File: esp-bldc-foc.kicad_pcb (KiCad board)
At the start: 4 copper layers, 66 x 66 mm, 94 parts, among them IC1 ESP32-S3FN8, IC2 LY68L6400SLIT, IC3 AS5600-ASOM, J1 USB_C_Receptacle_USB2.0, J10 UART, J3 I2C ENCODER, J6 Conn_01x02_Female, J7 A, J8 B, J9 C, Q1 BUK7M9R9-60EX, Q10 BUK7M9R9-60EX, Q11 BUK7M9R9-60EX, Q12 BUK7M9R9-60EX, Q2 BUK7M9R9-60EX, Q3 BUK7M9R9-60EX, Q4 BUK7M9R9-60EX, Q5 BUK7M9R9-60EX, Q6 BUK7M9R9-60EX, Q7 BUK7M9R9-60EX, Q8 BUK7M9R9-60EX, Q9 BUK7M9R9-60EX, SW1 SW_SPST, SW2 SW_SPST, U1 NCP163ASN330T1G, U2 DRV8353SMRTAT, U5 LMR36510ADDA, Y1 40MHz

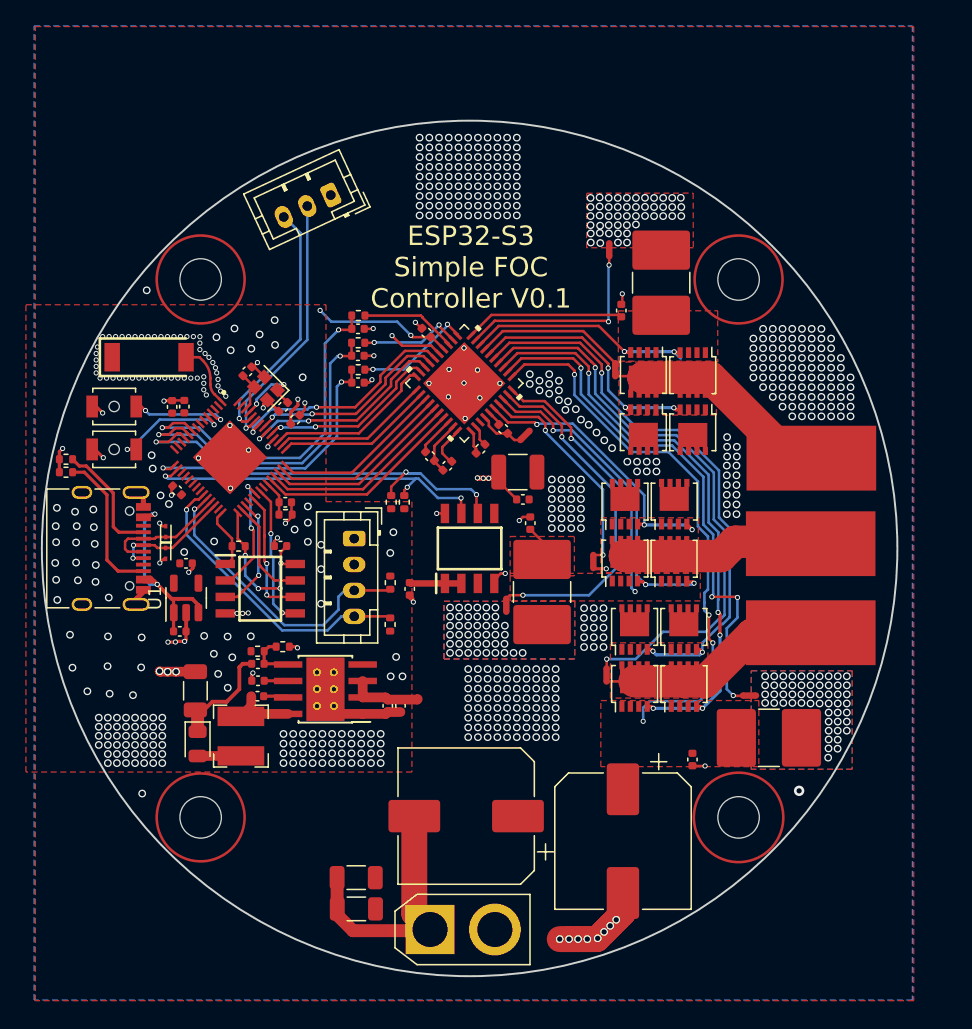
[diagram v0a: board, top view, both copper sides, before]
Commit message: init routing done
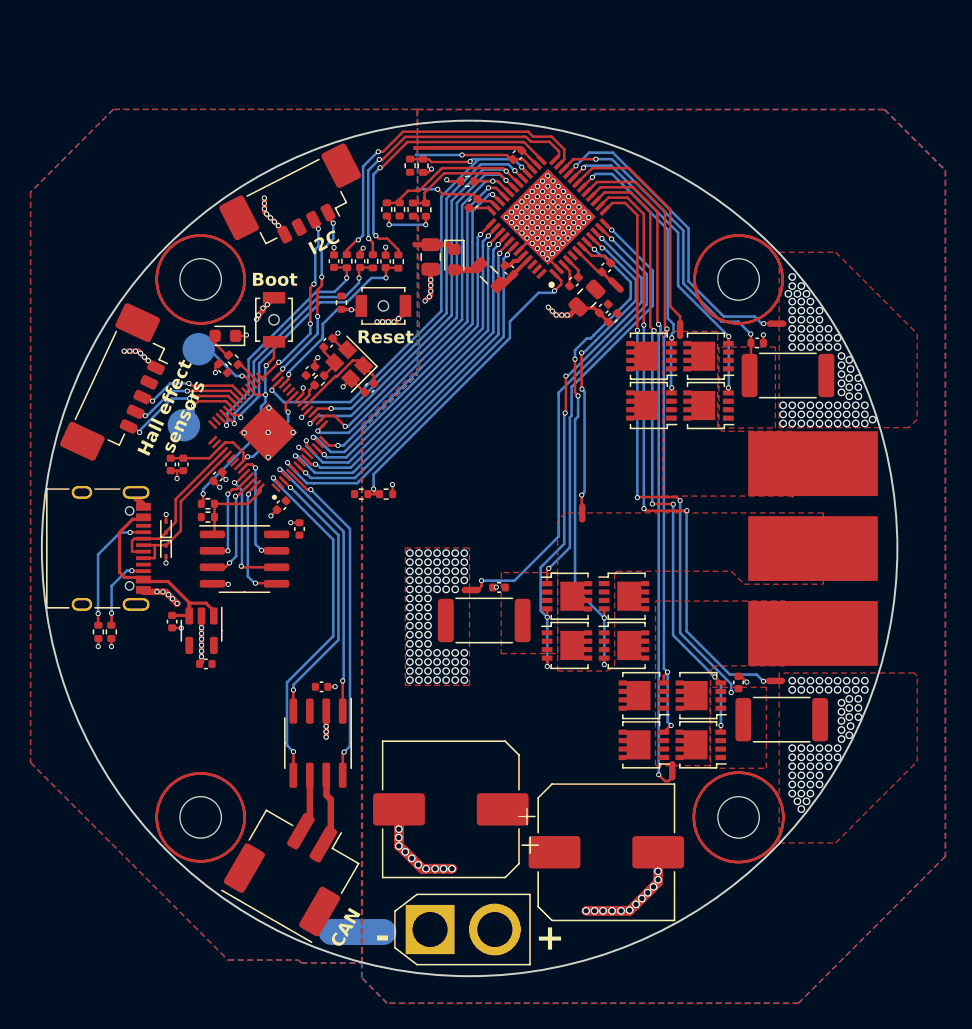
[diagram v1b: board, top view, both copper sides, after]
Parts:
- removed AE1: Antenna_Chip, 2450AT43F0100:ANTC6020X130N
- removed C32, C38: 1uF, Capacitor_SMD:C_0402_1005Metric
- removed C34, C36: 220nF, Capacitor_SMD:C_0402_1005Metric
- removed C40: 100nF, Capacitor_SMD:C_0402_1005Metric
- removed C42: 10pF, Capacitor_SMD:C_0402_1005Metric
- removed C44: 47uF, Capacitor_SMD:C_1206_3216Metric
- removed C46: 470uF, Capacitor_SMD:CP_Elec_10x10
- removed C49, C52: 4.7uF, Capacitor_SMD:C_1206_3216Metric
- removed D6: D, Diode_SMD:D_0805_2012Metric
- removed IC3: AS5600-ASOM, AS5600:SOIC127P600X175-8N
- removed J10: UART, Connector_JST:JST_PH_B3B-PH-K_1x03_P2.00mm_Vertical
- removed L4: 22uH, Inductor_SMD:L_Bourns-SRN4018
- removed R10, R11, R12, R9: 10K, Resistor_SMD:R_0402_1005Metric
- removed U5: LMR36510ADDA, Package_SO:Texas_HTSOP-8-1EP_3.9x4.9mm_P1.27mm_EP2.95x4.9mm_Mask2.4x3.1mm_ThermalVias
- added C24: 22uF, Capacitor_SMD:C_0805_2012Metric, F.Cu at (143.6, 78.5)
- added C25: C, Capacitor_SMD:C_0402_1005Metric, F.Cu at (135.2, 111.6)
- added C26: 0.1uF, Capacitor_SMD:C_0402_1005Metric, F.Cu at (124.5, 94.5)
- added C27: 1uF, Capacitor_SMD:C_0402_1005Metric, F.Cu at (123.5, 94.5)
- added C45: 470uF, Capacitor_SMD:CP_Elec_10x10, F.Cu at (157.2, 124.4)
- added D4: D, Diode_SMD:D_0603_1608Metric, F.Cu at (145.4, 78.7)
- added D5: LED, LED_SMD:LED_0603_1608Metric, F.Cu at (127.8, 84.5)
- added J2: Conn_01x05_Female, Connector_Molex:Molex_PicoBlade_53398-0571_1x05-1MP_P1.25mm_Vertical, F.Cu at (120.2, 88.7)
- added J4: Conn_01x04_Pin, Connector_Molex:Molex_PicoBlade_53398-0471_1x04-1MP_P1.25mm_Vertical, F.Cu at (133.4, 74.8)
- added L1: 15uH, Inductor_SMD:L_0805_2012Metric, F.Cu at (148.1, 79.8)
- added NT8: NetTie_2, NetTie:NetTie-2_SMD_Pad2.0mm, B.Cu at (138.0, 130.5)
- added R13: R, Resistor_SMD:R_0402_1005Metric, F.Cu at (136.7, 82.0)
- added R14: 1K, Resistor_SMD:R_0402_1005Metric, F.Cu at (135.0, 88.0)
- added R15: 75K, Resistor_SMD:R_0402_1005Metric, F.Cu at (142.2, 74.8)
- added R16: 75K, Resistor_SMD:R_0402_1005Metric, F.Cu at (143.2, 74.8)
- added R17: 28K, Resistor_SMD:R_0402_1005Metric, F.Cu at (138.2, 96.8)
- added R18: 8.45K, Resistor_SMD:R_0402_1005Metric, F.Cu at (140.2, 96.8)
- added R20: 47K, Resistor_SMD:R_0402_1005Metric, F.Cu at (146.4, 72.6)
- added R21: 75K, Resistor_SMD:R_0402_1005Metric, F.Cu at (141.2, 74.8)
- added R23: 75K, Resistor_SMD:R_0402_1005Metric, F.Cu at (140.2, 74.8)
- added R24: 10K, Resistor_SMD:R_0402_1005Metric, F.Cu at (142.0, 71.4)
- added TP1: TestPoint, TestPoint:TestPoint_Pad_D2.5mm, B.Cu at (125.7, 85.6)
- added TP2: TestPoint, TestPoint:TestPoint_Pad_D2.5mm, B.Cu at (124.6, 91.4)
- added U3: W25X40CLSN, Package_SO:SOIC-8_3.9x4.9mm_P1.27mm, F.Cu at (129.2, 101.8)
- C1: value 10uF -> 4.7uF; footprint Capacitor_SMD:C_1210_3225Metric -> Capacitor_SMD:C_0805_2012Metric
- C15: value 1uF -> 2.2uF
- C16: value 1uF -> 0.1uF
- C4: value 1uF -> 10pF
- C7: value 10nF -> 10pF
- C8: value 10nF -> 1uF
- IC1: value ESP32-S3FN8 -> RP2040; footprint esp32-s3:QFN40P700X700X90-57N-D -> RP2040:QFN40P700X700X90-57N-D
- IC2: value LY68L6400SLIT -> DRV8323RHRGZR; footprint LY68L6400SLIT:SOIC127P600X175-8N -> DRV8323:QFN50P700X700X100-49N-D
- J3: value I2C ENCODER -> Conn_01x02_Female; footprint Connector_JST:JST_PH_B4B-PH-K_1x04_P2.00mm_Vertical -> Connector_Molex:Molex_CLIK-Mate_502443-0270_1x02-1MP_P2.00mm_Vertical
- R1: value 442K -> 1K
- R19, R22, R8: footprint Resistor_SMD:R_2816_7142Metric -> Resistor_SMD:R_2512_6332Metric
- R25: value 100K -> 330
- R26: value 43.2K -> 330
- U2: value DRV8353SMRTAT -> MAX3051; footprint DRV8353M:DRV8353SMRTAT -> Package_SO:SOIC-8_3.9x4.9mm_P1.27mm
- Y1: value 40MHz -> Crystal_GND24_Small; footprint Crystal:Crystal_SMD_2016-4Pin_2.0x1.6mm -> Crystal:Crystal_SMD_2520-4Pin_2.5x2.0mm
- moved R25 39.6 mm to (143.0, 71.4), turned to -90 degrees
- moved IC2 36.3 mm to (152.7, 75.4), turned to 135 degrees
- moved U2 30.0 mm to (134.9, 116.0), turned to -90 degrees
- moved J3 25.6 mm to (133.2, 125.4), turned to 150 degrees
- moved R19 23.8 mm to (147.7, 106.5), turned to 180 degrees
- moved NT5 23.0 mm to (146.7, 104.2), turned to 180 degrees
- moved R26 22.5 mm to (128.4, 86.4), turned to -45 degrees
- moved SW1 22.2 mm to (140.0, 82.2), turned to 180 degrees
- moved C8 21.7 mm to (146.9, 74.3)
- moved NT3 21.6 mm to (170.2, 111.2), turned to 0 degrees
- moved R8 20.9 mm to (170.7, 114.2), turned to 0 degrees
- moved C21 20.2 mm to (167.3, 111.3)
- moved C22 20.0 mm to (148.9, 104.0), turned to 180 degrees
- moved Q1 18.7 mm to (160.1, 116.1), turned to 180 degrees
- moved NT2 17.3 mm to (162.2, 118.1), turned to 90 degrees
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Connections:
- C10 pad 2: GND -> GNDD
- C12 pad 1: GND -> GNDD
- C12 pad 2: /MCU/VDD_SPI -> +3.3V
- C13 pad 1: Net-(C13-Pad1) -> Net-(IC2-CPL)
- C13 pad 2: Net-(C13-Pad2) -> Net-(IC2-CPH)
- C14 pad 2: Net-(C14-Pad2) -> Net-(IC2-VDRAIN)
- C15 pad 1: Net-(C15-Pad1) -> VBUS
- C15 pad 2: Net-(C15-Pad2) -> GND
- C16 pad 1: Net-(C15-Pad2) -> Net-(IC2-SW)
- C16 pad 2: Net-(C16-Pad2) -> Net-(IC2-CB)
- C17 pad 2: GND -> GNDD
- C18 pad 1: /MCU/IO4 -> /MCU/ADC0
- C18 pad 2: GND -> GNDD
- C19 pad 1: /MCU/IO5 -> /MCU/ADC1
- C19 pad 2: GND -> GNDD
- C2 pad 2: GND -> GNDD
- C20 pad 1: /MCU/IO6 -> /MCU/ADC2
- C20 pad 2: GND -> GNDD
- C21 pad 1: /Power_stage/SN1 -> /Power_stage/SN2
- C22 pad 1: /Power_stage/SN2 -> /Power_stage/SN1
- C3 pad 2: GND -> GNDD
- C4 pad 2: GND -> GNDD
- C5 pad 2: GND -> GNDD
- C6 pad 2: GND -> GNDD
- C7 pad 1: /MCU/XTAL_N -> Net-(IC1-XIN)
- C7 pad 2: GND -> GNDD
- C8 pad 1: /MCU/XTAL_P -> Net-(IC2-DVDD)
- C8 pad 2: GND -> GNDD
- C9 pad 2: GND -> GNDD
- D2 pad 2: GND -> GNDD
- D3 pad 2: GND -> GNDD
- IC1 pad 1: Net-(AE1-Pad2) -> +3.3V
- IC1 pad 10: /MCU/IO5 -> +3.3V
- IC1 pad 11: /MCU/IO6 -> /MCU/IO8
- IC1 pad 12: /MCU/IO7 -> /MCU/IO9
- IC1 pad 13: /MCU/IO8 -> /MCU/IO10
- IC1 pad 14: /MCU/IO9 -> /MCU/IO11
- IC1 pad 15: /SCL -> /MCU/IO12
- IC1 pad 16: /SDA -> /MCU/IO13
- IC1 pad 17: /MCU/IO12 -> /MCU/IO14
- IC1 pad 18: /MCU/IO13 -> /MCU/IO15
- IC1 pad 19: /MCU/IO14 -> GNDD
- IC1 pad 2: +3.3V -> /CAN_SD
- IC1 pad 20: +3.3V -> Net-(IC1-XIN)
- IC1 pad 21: unconnected-(IC1-Pad21) -> Net-(IC1-XOUT)
- IC1 pad 22: unconnected-(IC1-Pad22) -> +3.3V
- IC1 pad 23: /EXT_SDA -> +1V2
- IC1 pad 24: /EXT_SCL -> unconnected-(IC1-SWCLK-Pad24)
- IC1 pad 25: /MCU/D_N -> unconnected-(IC1-SWDIO-Pad25)
- IC1 pad 26: /MCU/D_P -> /MCU/RESET
- IC1 pad 27: /MCU/IO21 -> /MCU/IO16
- IC1 pad 28: /MCU/SPICS1 -> /Encoder/I2C_SCL
- IC1 pad 29: /MCU/VDD_SPI -> /Encoder/I2C_SDA
- IC1 pad 3: +3.3V -> /UART_RX
- IC1 pad 30: /MCU/SPIHD -> /MCU/IO19
- IC1 pad 31: /MCU/SPIWP -> /MCU/TX0
- IC1 pad 32: /MCU/SPICS0 -> /MCU/USBBOOT
- IC1 pad 33: /MCU/SPICLK -> +3.3V
- IC1 pad 34: /MCU/SPIQ -> /Encoder/U
- IC1 pad 35: /MCU/SPID -> /Encoder/V
- IC1 pad 36: unconnected-(IC1-Pad36) -> /Encoder/W
- IC1 pad 37: Net-(C4-Pad1) -> /MCU/RX0
- IC1 pad 38: /MCU/IO33 -> /MCU/ADC0
- IC1 pad 39: /MCU/IO34 -> /MCU/ADC1
- IC1 pad 4: /MCU/RESET -> /UART_TX
- IC1 pad 40: /MCU/IO35 -> /MCU/ADC2
- IC1 pad 41: /MCU/IO36 -> /MCU/ADC3
- IC1 pad 42: /MCU/IO37 -> +3.3V
- IC1 pad 43: /MCU/IO38 -> +3.3V
- IC1 pad 44: /MCU/IO39 -> +3.3V
- IC1 pad 45: /MCU/IO40 -> +1V2
- IC1 pad 46: +3.3V -> /MCU/D_N
- IC1 pad 47: /MCU/IO41 -> /MCU/D_P
- IC1 pad 48: /MCU/IO42 -> +3.3V
- IC1 pad 49: /MCU/IO43 -> +3.3V
- IC1 pad 5: /MCU/IO0 -> /CAN_RS
- IC1 pad 50: /MCU/IO44 -> +1V2
- IC1 pad 51: /UART_TX -> /MCU/QSPI_D3
- IC1 pad 52: /UART_RX -> /MCU/QSPI_SCLK
- IC1 pad 53: /MCU/XTAL_N -> /MCU/QSPI_D0
- IC1 pad 54: /MCU/XTAL_P -> /MCU/QSPI_D2
- IC1 pad 55: +3.3V -> /MCU/QSPI_D1
- IC1 pad 56: +3.3V -> /MCU/QSPI_CS
- IC1 pad 57: GND -> GNDD
- IC1 pad 6: /MCU/IO1 -> /MCU/IO4
- IC1 pad 7: /MCU/IO2 -> /MCU/IO5
- IC1 pad 8: /MCU/IO3 -> /MCU/IO6
- IC1 pad 9: /MCU/IO4 -> /MCU/IO7
- IC2 pad 1: /MCU/SPICS1 -> /motor_controller/FB
- IC2 pad 2: /MCU/SPIQ -> GND
- IC2 pad 3: /MCU/SPIWP -> Net-(IC2-CPL)
- IC2 pad 4: GND -> Net-(IC2-CPH)
- IC2 pad 5: /MCU/SPID -> VBUS
- IC2 pad 6: /MCU/SPICLK -> /motor_controller/VDRAIN
- IC2 pad 7: /MCU/SPIHD -> Net-(IC2-VDRAIN)
- IC2 pad 8: /MCU/VDD_SPI -> /Power_stage/GHA
- J1 pad A1: GND -> GNDD
- J1 pad A12: GND -> GNDD
- J1 pad B1: GND -> GNDD
- J1 pad B12: GND -> GNDD
- J1 pad S1: GND -> GNDD
- J3 pad 1: +3.3V -> Net-(J3-Pin_1)
- J3 pad 2: GND -> Net-(J3-Pin_2)
- NT2 pad 1: /Power_stage/SHA -> /Power_stage/SHB
- NT2 pad 2: /Power_stage/A -> /Power_stage/B
- NT3 pad 1: /Power_stage/SP1 -> /Power_stage/SP2
- NT4 pad 1: /Power_stage/SHB -> /Power_stage/SHA
- NT4 pad 2: /Power_stage/B -> /Power_stage/A
- NT5 pad 1: /Power_stage/SP2 -> /Power_stage/SP1
- Q1 pad 1: /Power_stage/A -> /Power_stage/B
- Q1 pad 2: /Power_stage/A -> /Power_stage/B
- Q1 pad 3: /Power_stage/A -> /Power_stage/B
- Q1 pad 4: /Power_stage/GHA -> /Power_stage/GHB
- Q2 pad 1: /Power_stage/SN1 -> /Power_stage/SN2
- Q2 pad 2: /Power_stage/SN1 -> /Power_stage/SN2
- Q2 pad 3: /Power_stage/SN1 -> /Power_stage/SN2
- Q2 pad 4: /Power_stage/GLA -> /Power_stage/GLB
- Q2 pad 5: /Power_stage/A -> /Power_stage/B
- Q3 pad 1: /Power_stage/A -> /Power_stage/B
- Q3 pad 2: /Power_stage/A -> /Power_stage/B
- Q3 pad 3: /Power_stage/A -> /Power_stage/B
- Q3 pad 4: /Power_stage/GHA -> /Power_stage/GHB
- Q4 pad 1: /Power_stage/SN1 -> /Power_stage/SN2
- Q4 pad 2: /Power_stage/SN1 -> /Power_stage/SN2
- Q4 pad 3: /Power_stage/SN1 -> /Power_stage/SN2
- Q4 pad 4: /Power_stage/GLA -> /Power_stage/GLB
- Q4 pad 5: /Power_stage/A -> /Power_stage/B
- Q5 pad 1: /Power_stage/B -> /Power_stage/A
- Q5 pad 2: /Power_stage/B -> /Power_stage/A
- Q5 pad 3: /Power_stage/B -> /Power_stage/A
- Q5 pad 4: /Power_stage/GHB -> /Power_stage/GHA
- Q6 pad 1: /Power_stage/SN2 -> /Power_stage/SN1
- Q6 pad 2: /Power_stage/SN2 -> /Power_stage/SN1
- Q6 pad 3: /Power_stage/SN2 -> /Power_stage/SN1
- Q6 pad 4: /Power_stage/GLB -> /Power_stage/GLA
- Q6 pad 5: /Power_stage/B -> /Power_stage/A
- Q7 pad 1: /Power_stage/B -> /Power_stage/A
- Q7 pad 2: /Power_stage/B -> /Power_stage/A
- Q7 pad 3: /Power_stage/B -> /Power_stage/A
- Q7 pad 4: /Power_stage/GHB -> /Power_stage/GHA
- Q8 pad 1: /Power_stage/SN2 -> /Power_stage/SN1
- Q8 pad 2: /Power_stage/SN2 -> /Power_stage/SN1
- Q8 pad 3: /Power_stage/SN2 -> /Power_stage/SN1
- Q8 pad 4: /Power_stage/GLB -> /Power_stage/GLA
- Q8 pad 5: /Power_stage/B -> /Power_stage/A
- R1 pad 1: Net-(C4-Pad1) -> /MCU/QSPI_CS
- R1 pad 2: GND -> /MCU/USBBOOT
- R19 pad 1: /Power_stage/SN2 -> /Power_stage/SN1
- R2 pad 1: /MCU/VDD_SPI -> +3.3V
- R2 pad 2: /MCU/SPICS1 -> /MCU/QSPI_CS
- R25 pad 1: +3.3V -> /MCU/IO16
- R25 pad 2: Net-(C42-Pad2) -> GND
- R26 pad 1: Net-(C42-Pad2) -> Net-(D5-A)
- R26 pad 2: GND -> /MCU/IO19
- R3 pad 1: Net-(R3-Pad1) -> Net-(IC2-SOA)
- R3 pad 2: /MCU/IO4 -> /MCU/ADC0
- R4 pad 1: GND -> GNDD
- R5 pad 1: GND -> GNDD
- R6 pad 1: Net-(R6-Pad1) -> Net-(IC2-SOB)
- R6 pad 2: /MCU/IO5 -> /MCU/ADC1
- R7 pad 1: Net-(R7-Pad1) -> Net-(IC2-SOC)
- R7 pad 2: /MCU/IO6 -> /MCU/ADC2
- R8 pad 1: /Power_stage/SN1 -> /Power_stage/SN2
- SW1 pad 1: GND -> GNDD
- SW2 pad 1: GND -> GNDD
- SW2 pad 2: /MCU/IO0 -> /MCU/USBBOOT
- U1 pad 2: GND -> GNDD
- U2 pad 1: Net-(C13-Pad1) -> /UART_TX
- U2 pad 2: Net-(C13-Pad2) -> GNDD
- U2 pad 3: VBUS -> +3.3V
- U2 pad 4: /motor_controller/VDRAIN -> /UART_RX
- U2 pad 5: Net-(C14-Pad2) -> /CAN_SD
- U2 pad 6: /Power_stage/GHA -> Net-(J3-Pin_2)
- U2 pad 7: /Power_stage/SHA -> Net-(J3-Pin_1)
- U2 pad 8: /Power_stage/GLA -> /CAN_RS
- Y1 pad 1: /MCU/XTAL_N -> Net-(IC1-XIN)
- Y1 pad 2: GND -> GNDD
- Y1 pad 3: /MCU/XTAL_P -> Net-(C4-Pad1)
- Y1 pad 4: GND -> GNDD
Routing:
- net GNDD: track 0.00 -> 55.9 mm, vias 0 -> 63
- net /MCU/IO14: track 0.00 -> 41.1 mm, vias 0 -> 2
- net /MCU/IO16: track 0.00 -> 39.9 mm, vias 0 -> 3
- net GND: track 78.2 -> 39.2 mm, vias 272 -> 341
- net /MCU/IO13: track 0.00 -> 37.9 mm, vias 0 -> 2
- net /SCL: track 30.9 -> 0.00 mm, vias 3 -> 0
- net /MCU/IO12: track 0.00 -> 30.5 mm, vias 0 -> 2
- net /MCU/IO15: track 0.00 -> 29.8 mm, vias 0 -> 2
- net /MCU/IO10: track 0.00 -> 29.2 mm, vias 0 -> 2
- net /MCU/IO8: track 0.00 -> 28.0 mm, vias 0 -> 2
- net /MCU/IO11: track 0.00 -> 27.8 mm, vias 0 -> 2
- net /SDA: track 27.7 -> 0.00 mm, vias 3 -> 0
- net /CAN_SD: track 0.00 -> 27.2 mm, vias 0 -> 2
- net /MCU/IO7: track 0.00 -> 26.7 mm, vias 0 -> 2
- net Net-(IC2-SOC): track 0.00 -> 25.9 mm, vias 0 -> 2
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- added copper zone on B.Cu, net GNDD
- added copper zone on In2.Cu, net GNDD
- removed copper zone on In1.Cu, net /Power_stage/SN1
- removed copper zone on In2.Cu, net /Power_stage/SN1
- removed copper zone on In1.Cu, net GND
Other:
- board text added: "+"
- board text added: "-"
- board text added: "Boot"
- board text added: "CAN"
- board text added: "Hall effect sensors"
- board text added: "I2C"
- board text added: "RP2040 Simple FOC Controller"
- board text added: "RX"
- board text added: "Reset"
- board text added: "TX"
- board text added: "V1.0"
- board text removed: "ESP32-S3 Simple FOC Controller V0.1"
- board text removed: "Made By: Keion Bisland Sep 2, 2022"
